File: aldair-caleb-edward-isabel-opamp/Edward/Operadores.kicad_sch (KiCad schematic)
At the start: 50 parts, among them J1 Conn_01x01_Pin, J10 Conn_01x01_Pin, J11 Conn_01x01_Pin, J12 Conn_01x01_Pin, J13 Conn_01x01_Pin, J14 Conn_01x01_Pin, J15 Conn_01x01_Pin, J16 Conn_01x01_Pin, J2 Conn_01x01_Pin, J3 Conn_01x01_Pin, J4 Conn_01x01_Pin, J5 Conn_01x01_Pin, J6 Conn_01x01_Pin, J7 Conn_01x01_Pin, J8 Conn_01x01_Pin, J9 Conn_01x01_Pin, U1 LM741, U2 LM741, U3 LM741, U4 LM741, U5 LM741, U6 LM741, U7 LM741, U8 LM741

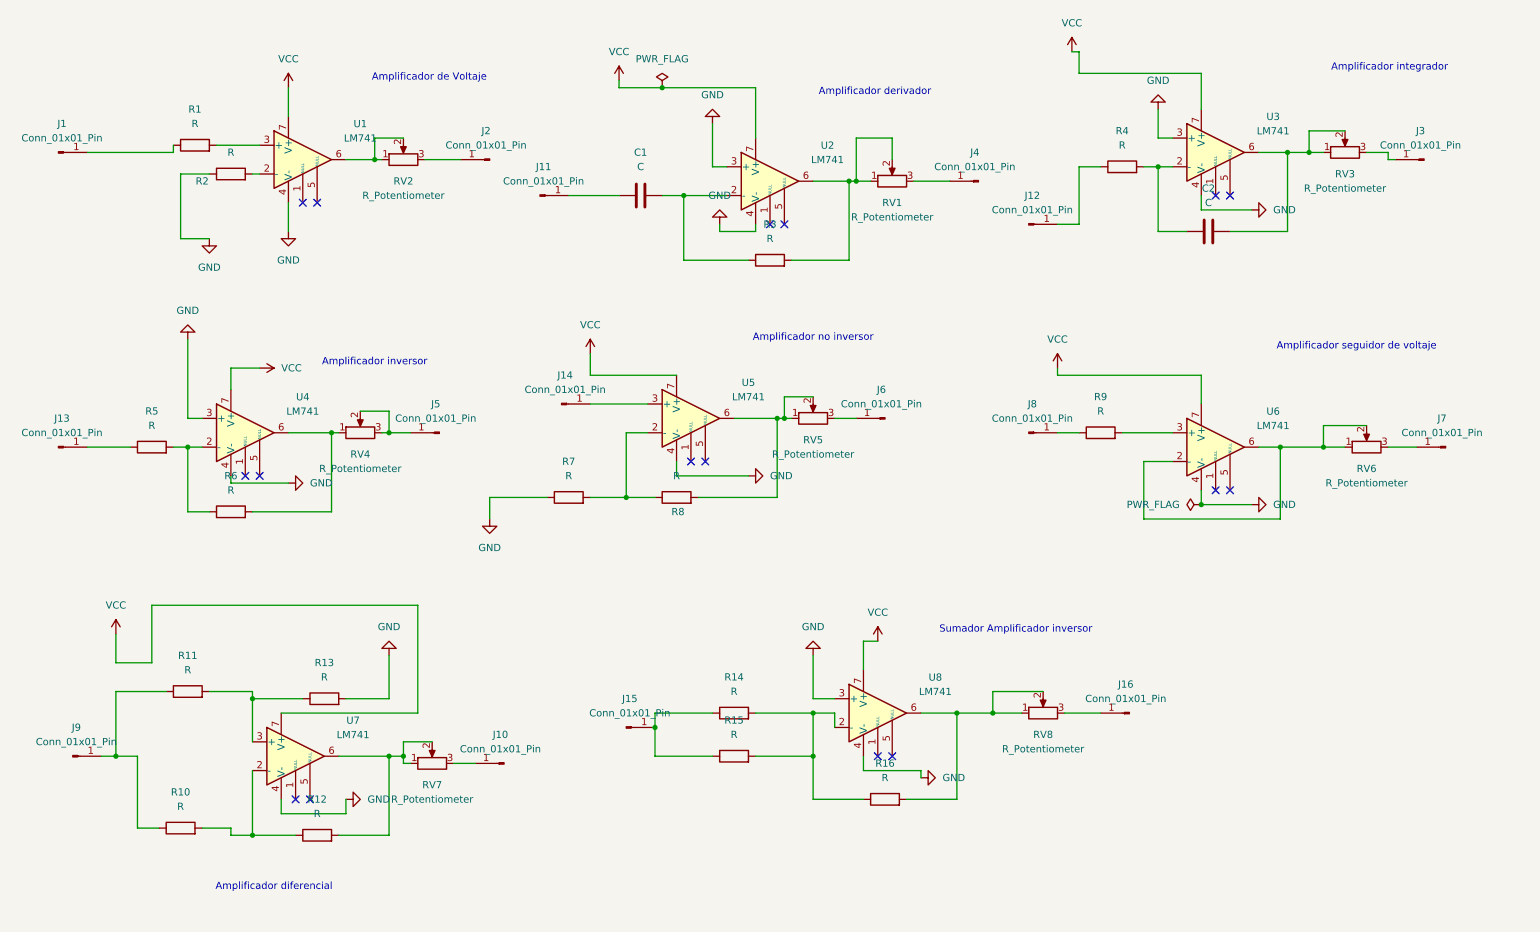
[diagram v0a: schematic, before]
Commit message: Cambios Finales Prueba OP AMP - EDWARDS
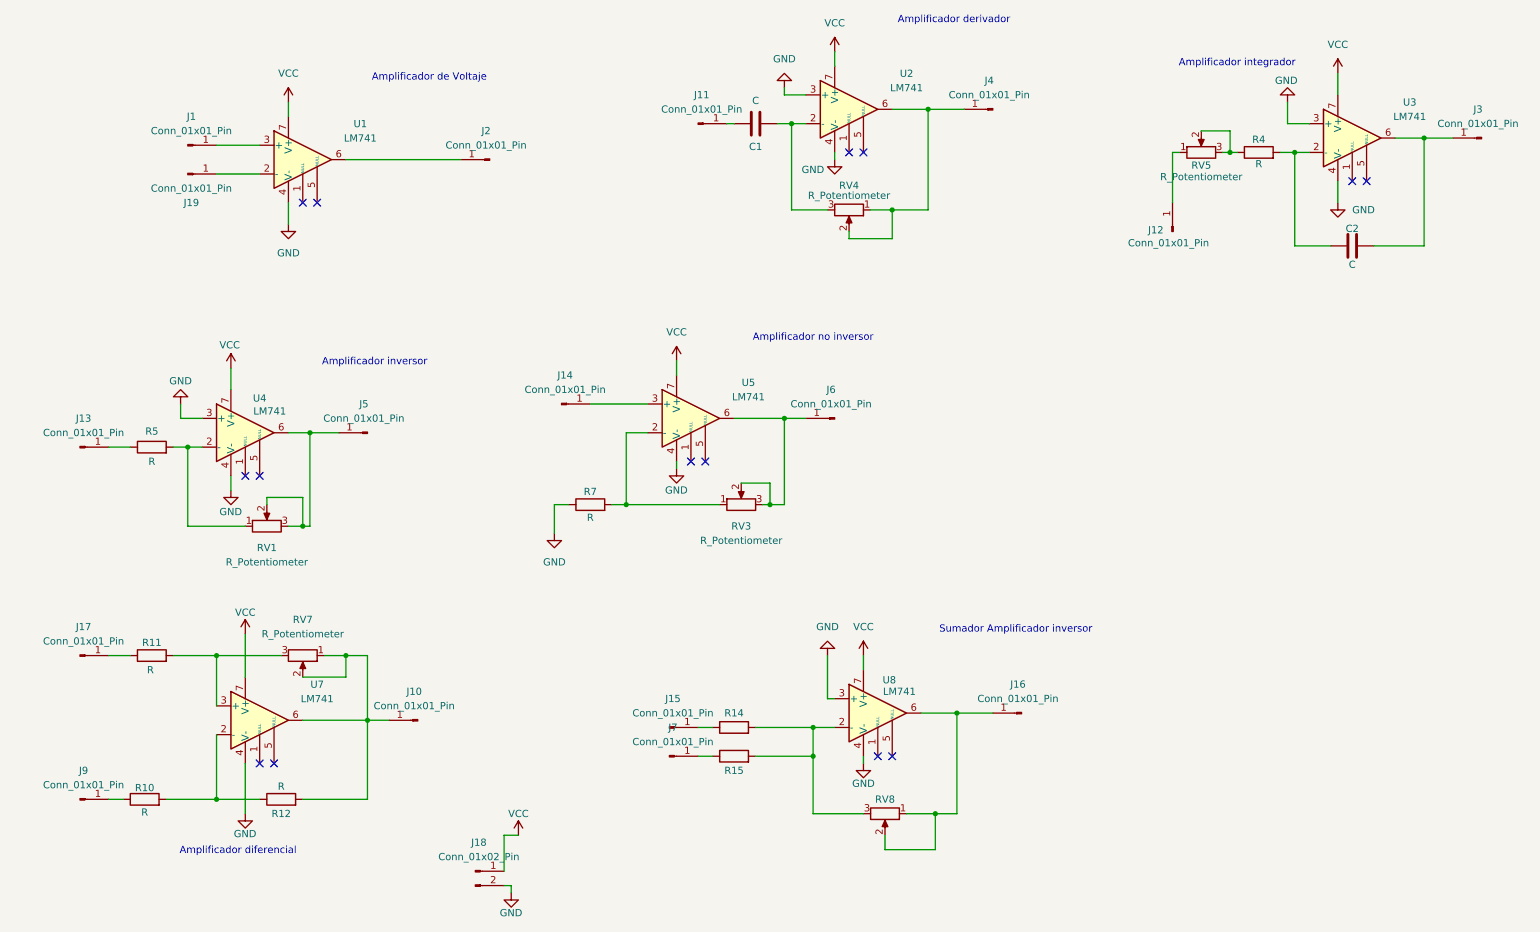
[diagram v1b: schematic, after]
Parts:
- removed J8: Conn_01x01_Pin, Connector_PinSocket_2.54mm:PinSocket_1x01_P2.54mm_Vertical, symbol Connector:Conn_01x01_Pin
- removed R1, R13, R16, R2, R3, R6, R8, R9: R, Resistor_THT:R_Axial_DIN0207_L6.3mm_D2.5mm_P10.16mm_Horizontal, symbol Device:R
- removed RV2, RV6: R_Potentiometer, Potentiometer_THT:Potentiometer_Bourns_3266Z_Horizontal, symbol Device:R_Potentiometer
- removed U6: LM741, Package_DIP:DIP-6_W7.62mm_LongPads, symbol Amplifier_Operational:LM741
- added J17, J19: Conn_01x01_Pin, Connector_PinSocket_2.54mm:PinSocket_1x01_P2.54mm_Vertical, symbol Connector:Conn_01x01_Pin
- added J18: Conn_01x02_Pin, Connector_PinHeader_2.54mm:PinHeader_1x02_P2.54mm_Vertical, symbol Connector:Conn_01x02_Pin
- RV1, RV3, RV4, RV5, RV7, RV8: footprint Potentiometer_THT:Potentiometer_Bourns_3266Z_Horizontal -> Potentiometer_THT:Potentiometer_Omeg_PC16BU_Vertical
- U1: footprint Package_DIP:DIP-6_W10.16mm -> Package_DIP:DIP-8_W7.62mm_Socket_LongPads
- U2, U3: footprint Package_DIP:DIP-6_W7.62mm -> Package_DIP:DIP-8_W7.62mm_Socket_LongPads
- U4, U5, U7, U8: footprint Package_DIP:DIP-6_W7.62mm_LongPads -> Package_DIP:DIP-8_W7.62mm_Socket_LongPads
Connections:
- net GND: now also J18.2 (Pin_2)
- net VCC: now also J18.1 (Pin_1)
- net at J10.1 (Pin_1): now also R12.2, RV7.1, RV7.2, U7.6; no longer RV7.3
- net at RV4.1: now also J4.1 (Pin_1), RV4.2, U2.6; no longer U4.6
- net at R11.2, U7.3 (+): now also RV7.3
- net at J7.1 (Pin_1): now also R15.1
- net at J15.1 (Pin_1), R14.1: no longer R15.1
- net at R14.2, R15.2, U8.2 (-): now also RV8.3
- net at RV8.1, RV8.2, U8.6: now also J16.1 (Pin_1)
- net at RV1.3: now also J5.1 (Pin_1), RV1.2, U4.6; no longer J4.1 (Pin_1)
- net at J9.1 (Pin_1), R10.1: no longer R11.1
- net at R7.2, U5.2 (-): now also RV3.1
- net at J1.1 (Pin_1): now also U1.3 (+)
- net at J12.1 (Pin_1): now also RV5.1; no longer R4.1
- net at R5.2, U4.2 (-): now also RV1.1
- net at C2.2, U3.6: now also J3.1 (Pin_1); no longer RV3.1, RV3.2
- net at RV3.3: now also J6.1 (Pin_1), RV3.2, U5.6; no longer J3.1 (Pin_1)
- net at J2.1 (Pin_1): now also U1.6
- net at RV5.3: now also R4.1, RV5.2; no longer J6.1 (Pin_1)
- net at U1.2 (-): now also J19.1 (Pin_1)
- net at C1.2, U2.2 (-): now also RV4.3
- new net: J17.1 (Pin_1), R11.1
- no-connect marks 16 -> 14
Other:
- note removed: "Amplificador seguidor de voltaje"
- moved on the sheet: C1, C2, J1, J10, J11, J12, J13, J15, J16, J3, J4, J5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
